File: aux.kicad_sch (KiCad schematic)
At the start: 4 parts

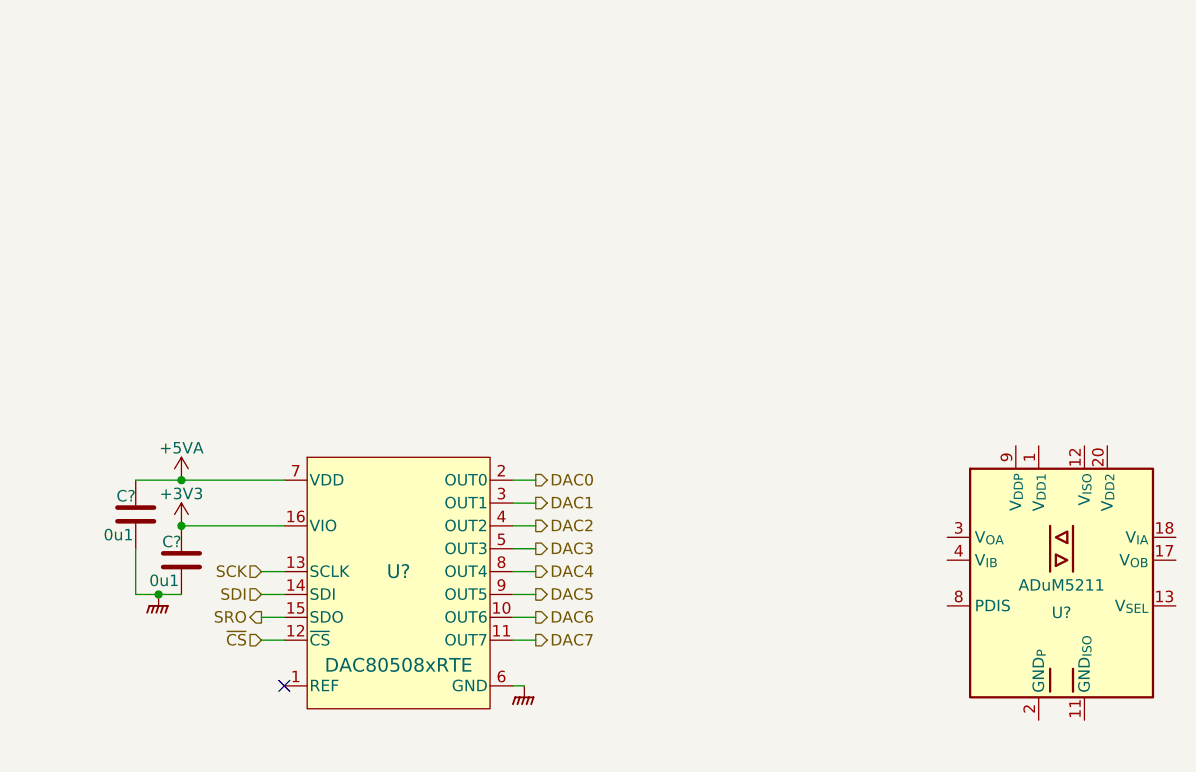
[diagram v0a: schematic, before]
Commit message: Schematic complete, maybe
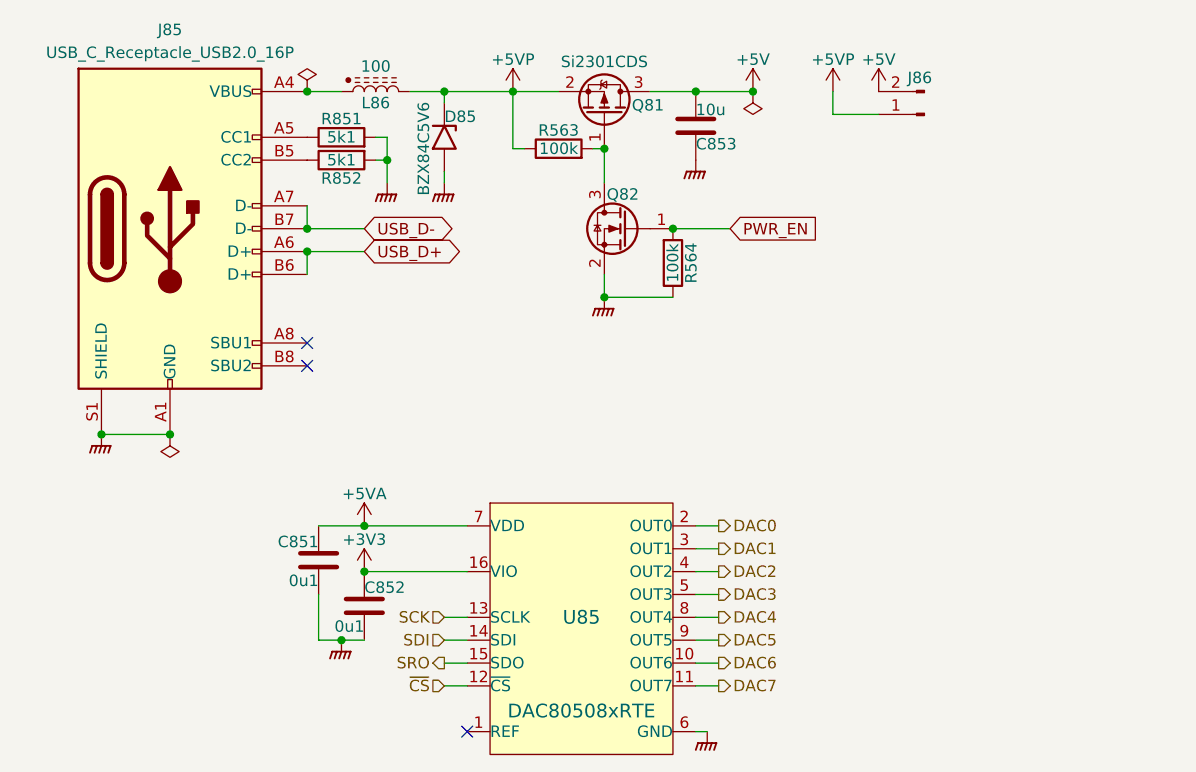
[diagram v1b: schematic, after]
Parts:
- removed U?: ADuM5211, Package_SO:SSOP-20_5.3x7.2mm_P0.65mm, symbol Isolator:ADuM5211
- added C853: 10u, Capacitor_SMD:C_0603_1608Metric, symbol Device:C
- added D85: BZX84C5V6, Package_TO_SOT_SMD:SOT-23, symbol Parts:BZX84Cxx
- added J85: USB_C_Receptacle_USB2.0_16P, symbol Connector:USB_C_Receptacle_USB2.0_16P
- added J86: Conn_01x02_Pin, symbol Connector:Conn_01x02_Pin
- added L86: 100, Inductor_SMD:L_0603_1608Metric, symbol Parts:L_Ferrite_Power
- added Q81: Si2301CDS, Package_TO_SOT_SMD:SOT-23, symbol External:Si2301CDS
- added Q82: AO3400A, Package_TO_SOT_SMD:SOT-23, symbol Transistor_FET:AO3400A
- added R563, R564: 100k, symbol Device:R
- added R851, R852: 5k1, symbol Device:R
- C851, C852: renamed from C?; LCSC (none) -> C307331
- U85: renamed from U?; footprint RTE0016D -> Package_DFN_QFN:Texas_RTE0016D_WQFN-16-1EP_3x3mm_P0.5mm_EP0.8x0.8mm; LCSC (none) -> C2863226
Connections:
- net GNDPWR: now also C853.2, D85.1 (A), J85.A1 (GND), J85.A12 (GND), J85.B1 (GND), J85.B12 (GND), J85.S1 (SHIELD), Q82.2 (S), R564.1, R851.2, R852.2
- new net: Q81.1 (G), Q82.3 (D), R563.2
- new net: J85.A5 (CC1), R851.1
- new net: J85.B5 (CC2), R852.1
- new net: J85.A4 (VBUS), J85.A9 (VBUS), J85.B4 (VBUS), J85.B9 (VBUS), L86.1
- new net +5V: C853.1, J86.2 (Pin_2), Q81.3 (D)
- new net +5VP: D85.3 (K), J86.1 (Pin_1), L86.2, Q81.2 (S), R563.1
- new net PWR_EN: Q82.1 (G), R564.2
- new net USB_D+: J85.A6 (D+), J85.B6 (D+)
- new net USB_D-: J85.A7 (D-), J85.B7 (D-)
- no-connect marks 1 -> 3
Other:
- moved on the sheet: C851, C852, U85

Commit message: Part selection
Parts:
- J85, J86: now left out of the parts list
- Q81: LCSC (none) -> C10487
- Q82: LCSC (none) -> C20917
- R563, R564: footprint (none) -> Resistor_SMD:R_0402_1005Metric; LCSC (none) -> C25741
- R851, R852: footprint (none) -> Resistor_SMD:R_0402_1005Metric; LCSC (none) -> C25905
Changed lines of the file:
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@@
+			)
+		)
+		(property "LCSC" "C10487"
+			(at 129.54 29.21 90)
+			(effects
+				(font
+					(size 1.27 1.27)
+				)
+				(hide yes)
 			)
 		)
@@
 			)
 		)
-		(property "Footprint" ""
+		(property "Footprint" "Resistor_SMD:R_0402_1005Metric"
 			(at 100.33 33.528 90)
 			(effects
@@
 			)
 		)
+		(property "LCSC" "C25905"
+			(at 100.33 31.75 90)
+			(effects
+				(font
+					(size 1.27 1.27)
+				)
+				(hide yes)
+			)
+		)
 		(pin "1"
 		)
@@
 			)
 		)
-		(property "Footprint" ""
+		(property "Footprint" "Resistor_SMD:R_0402_1005Metric"
 			(at 124.46 34.798 90)
 			(effects
@@
 		(property "Description" "Resistor"
 			(at 124.46 33.02 0)
+			(effects
+				(font
+					(size 1.27 1.27)
+				)
+				(hide yes)
+			)
+		)
+		(property "LCSC" "C25741"
+			(at 124.46 33.02 90)
 			(effects
 				(font
@@
 			)
 		)
-		(property "Footprint" ""
+		(property "Footprint" "Resistor_SMD:R_0402_1005Metric"
 			(at 100.33 32.512 90)
 			(effects
@@
 			)
 		)
+		(property "LCSC" "C25905"
+			(at 100.33 34.29 90)
+			(effects
+				(font
+					(size 1.27 1.27)
+				)
+				(hide yes)
+			)
+		)
 		(pin "1"
 		)
@@
 		(unit 1)
 		(exclude_from_sim no)
-		(in_bom yes)
+		(in_bom no)
 		(on_board yes)
 		(dnp no)
@@
 		(unit 1)
 		(exclude_from_sim no)
-		(in_bom yes)
+		(in_bom no)
 		(on_board yes)
 		(dnp no)
@@
 			)
 		)
+		(property "LCSC" "C20917"
+			(at 132.08 41.91 0)
+			(effects
+				(font
+					(size 1.27 1.27)
+				)
+				(hide yes)
+			)
+		)
 		(pin "1"
 		)
@@
 			)
 		)
-		(property "Footprint" ""
+		(property "Footprint" "Resistor_SMD:R_0402_1005Metric"
 			(at 135.382 45.72 90)
 			(effects
@@
 			(effects
 				(font
+					(size 1.27 1.27)
+				)
+				(hide yes)
+			)
+		)
+		(property "LCSC" "C25741"
+			(at 137.16 45.72 90)
+			(effects
+				(font
